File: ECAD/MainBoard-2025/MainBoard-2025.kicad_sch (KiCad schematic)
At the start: 62 parts, among them J1 XT60, J11 Conn_01x04, J12 Conn_01x04, J15 Conn_01x02, J16 XT30, J18 Conn_01x02, J2 Conn_01x04, J20 BAU, J21 BAU, J22 Conn_01x04, J23 Conn_01x02, J26 BAU, J28 Conn_01x02, J4 Conn_01x02, J6 Conn_01x06, J7 XT30, J8 Conn_01x02, J9 Conn_01x02, K2 FINDER-36.11, U2 R-78B3.3-2.0, U3 R-78B12-2.0, U4 R-78B5.0-2.0, U5 Teensy4.1

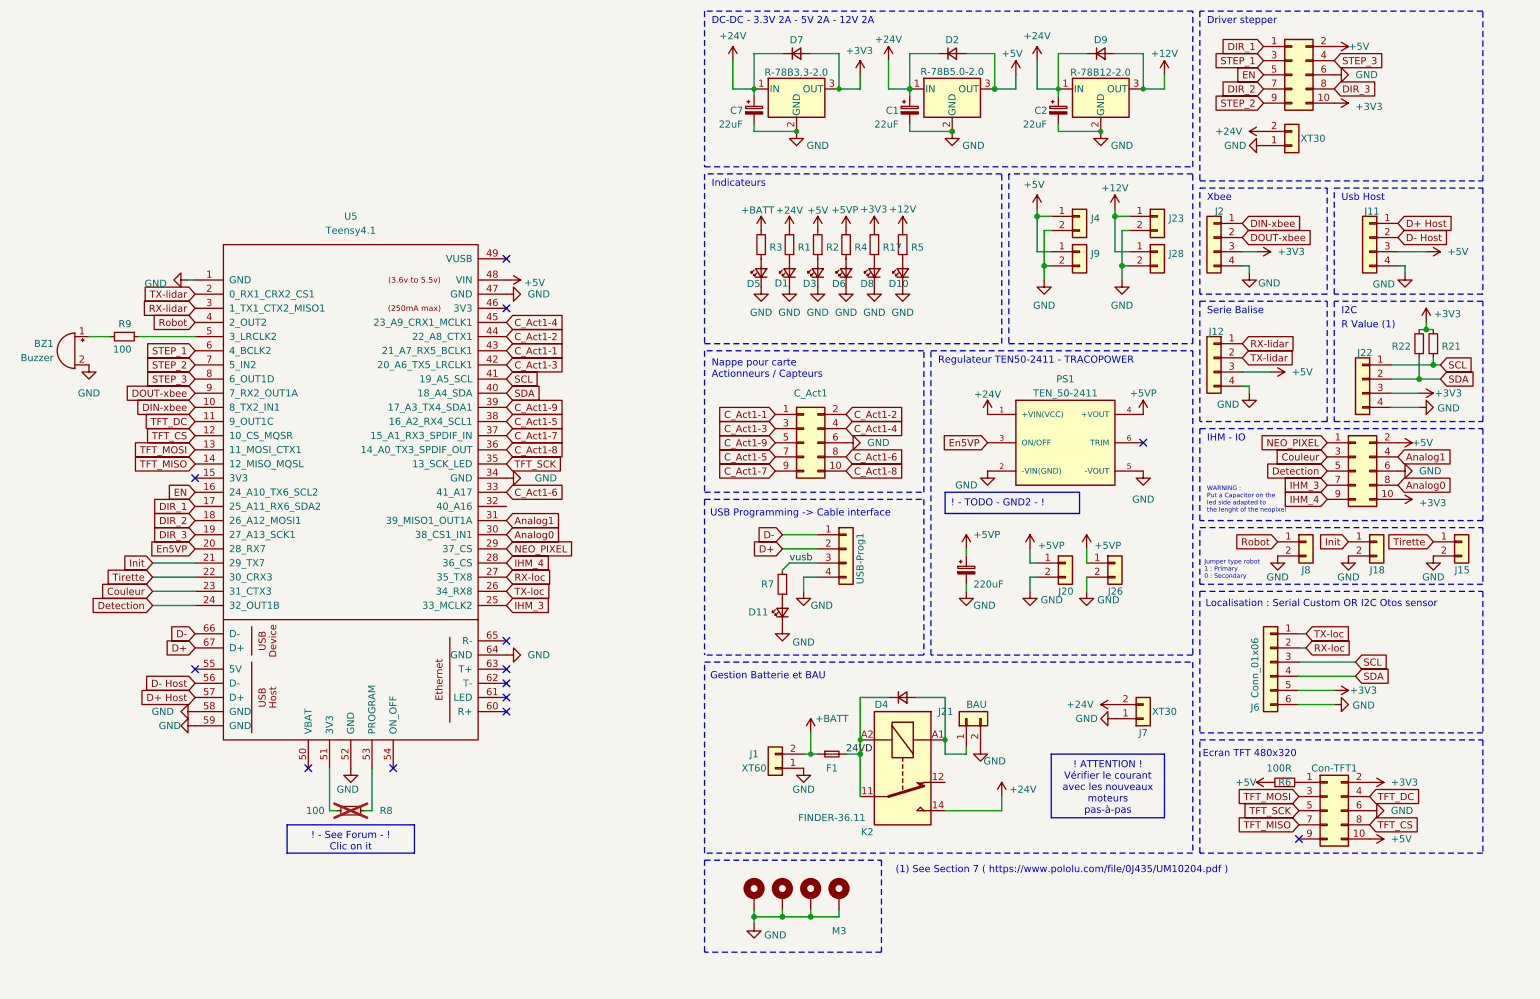
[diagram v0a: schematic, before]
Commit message: Power all the components
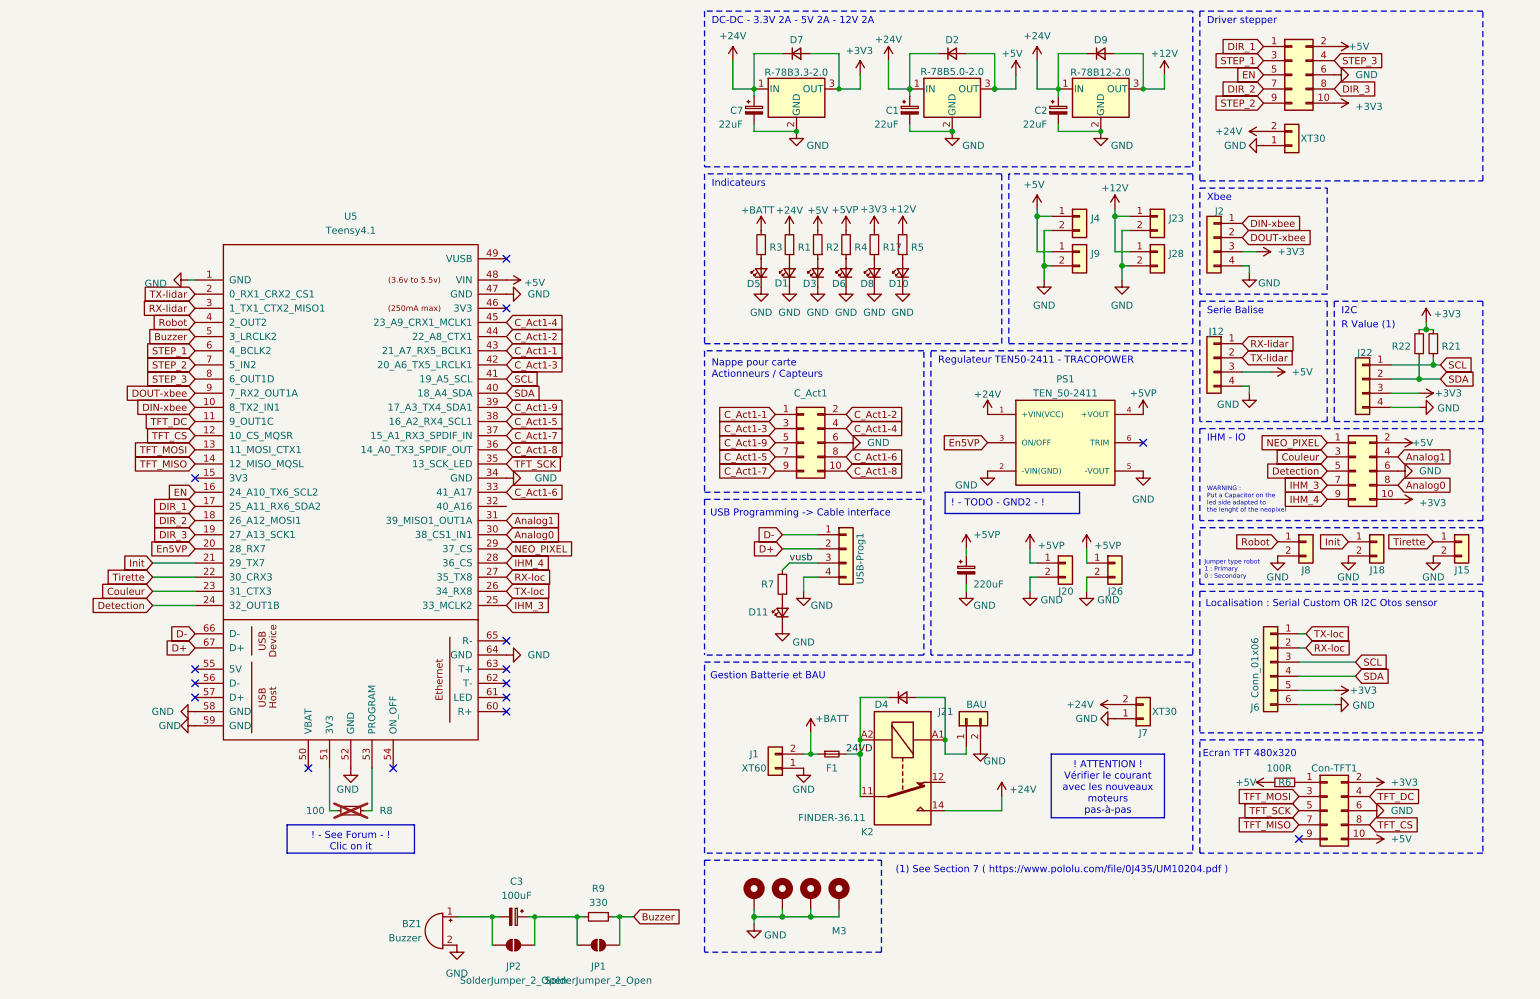
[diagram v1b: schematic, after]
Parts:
- removed J11: Conn_01x04, Connector_Molex:Molex_KK-254_AE-6410-04A_1x04_P2.54mm_Vertical, symbol Connector_Generic:Conn_01x04
- added C3: 100uF, Capacitor_SMD:CP_Elec_5x5.4, symbol Device:CP_Small
- added JP1, JP2: SolderJumper_2_Open, Jumper:SolderJumper-2_P1.3mm_Open_RoundedPad1.0x1.5mm, symbol Jumper:SolderJumper_2_Open
- BZ1: footprint (none) -> Buzzer_Beeper:Buzzer_15x7.5RM7.6
- R9: value 100 -> 330
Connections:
- net Buzzer: now reaches R9.1, U5.5 (3_LRCLK2)
- net Buzzer: now also JP1.2 (B)
- net at BZ1.1 (+): now also C3.2, JP2.1 (A); no longer R9.2
- net D+ Host: no longer names the net of U5.57 (D+)
- net D- Host: no longer names the net of U5.56 (D-)
- new net: C3.1, JP1.1 (A), JP2.2 (B), R9.2
- no-connect marks 13 -> 15
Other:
- note removed: "Usb Host"

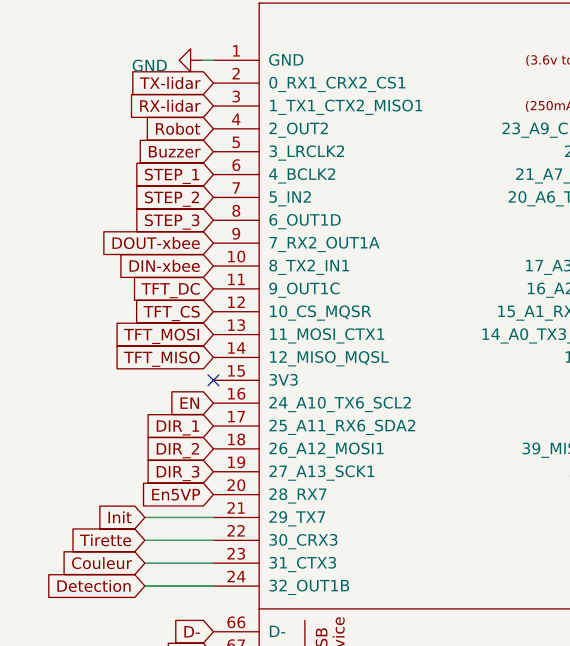
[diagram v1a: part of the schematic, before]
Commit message: Routing ok - Just before Silkscreen
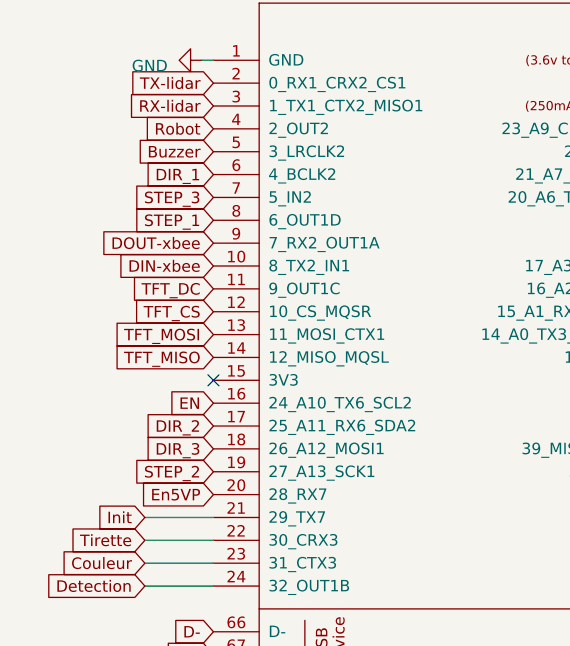
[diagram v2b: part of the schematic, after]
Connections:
- net DIR_1: now also U5.6 (4_BCLK2); no longer U5.17 (25_A11_RX6_SDA2)
- net DIR_2: now also U5.17 (25_A11_RX6_SDA2); no longer U5.18 (26_A12_MOSI1)
- net DIR_3: now also U5.18 (26_A12_MOSI1); no longer U5.19 (27_A13_SCK1)
- net STEP_1: now also U5.8 (6_OUT1D); no longer U5.6 (4_BCLK2)
- net STEP_2: now also U5.19 (27_A13_SCK1); no longer U5.7 (5_IN2)
- net STEP_3: now also U5.7 (5_IN2); no longer U5.8 (6_OUT1D)
